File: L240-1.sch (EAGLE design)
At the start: 13 parts, among them IC1 TINY13-20SSU, IC2 LM1117IMPX-3.3, X2 22-23-2021, X3 MKDSN1,5/6-5,08

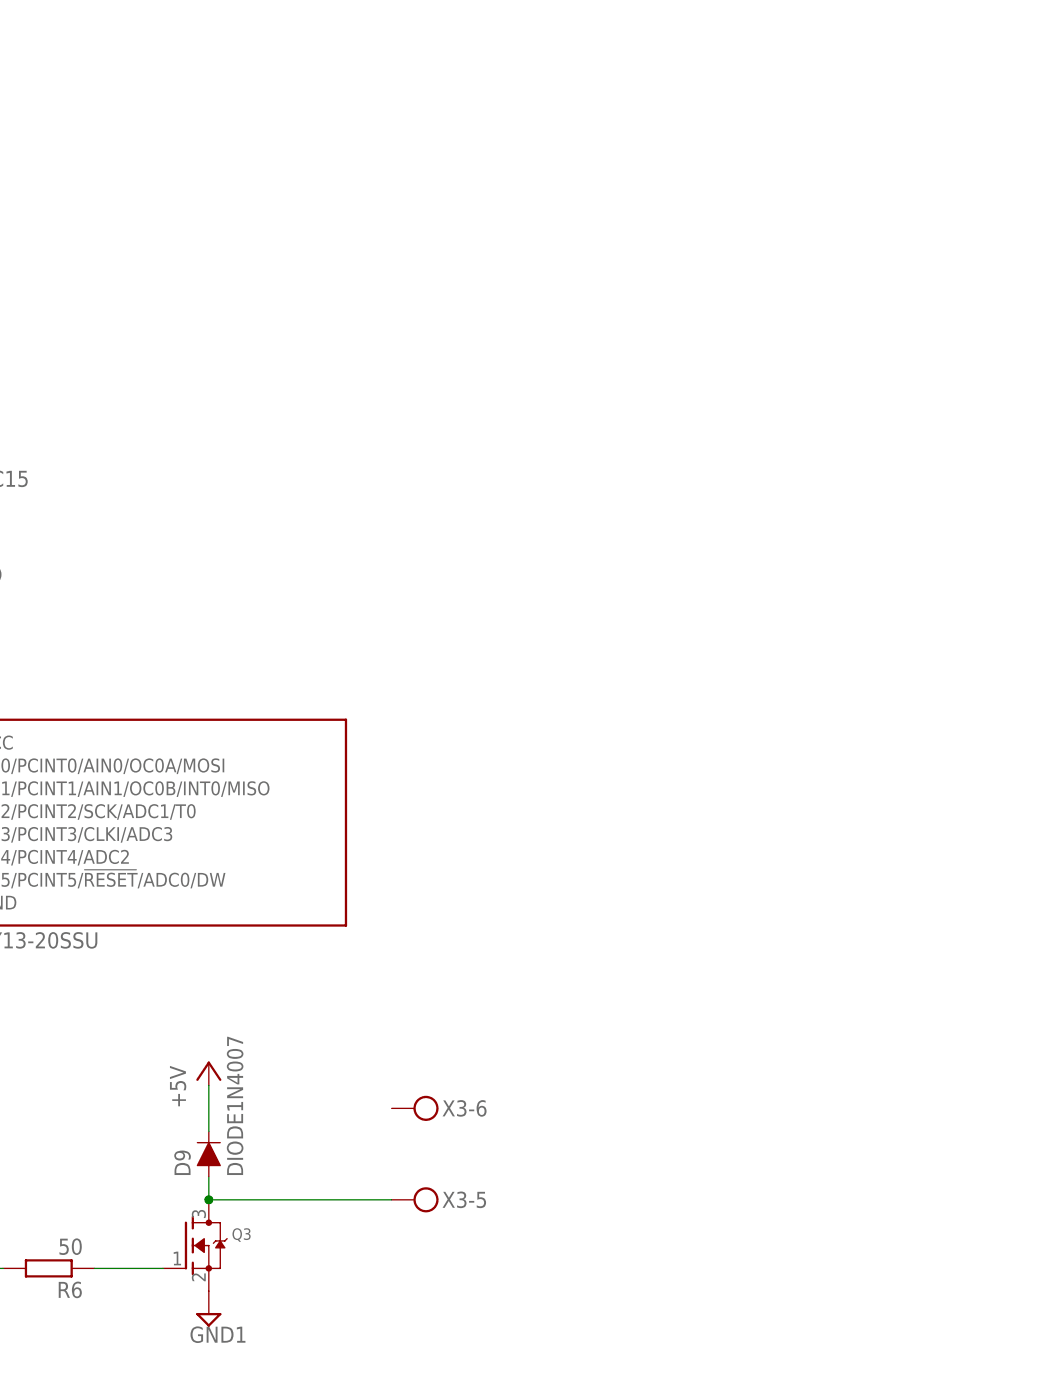
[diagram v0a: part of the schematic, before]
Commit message: relay
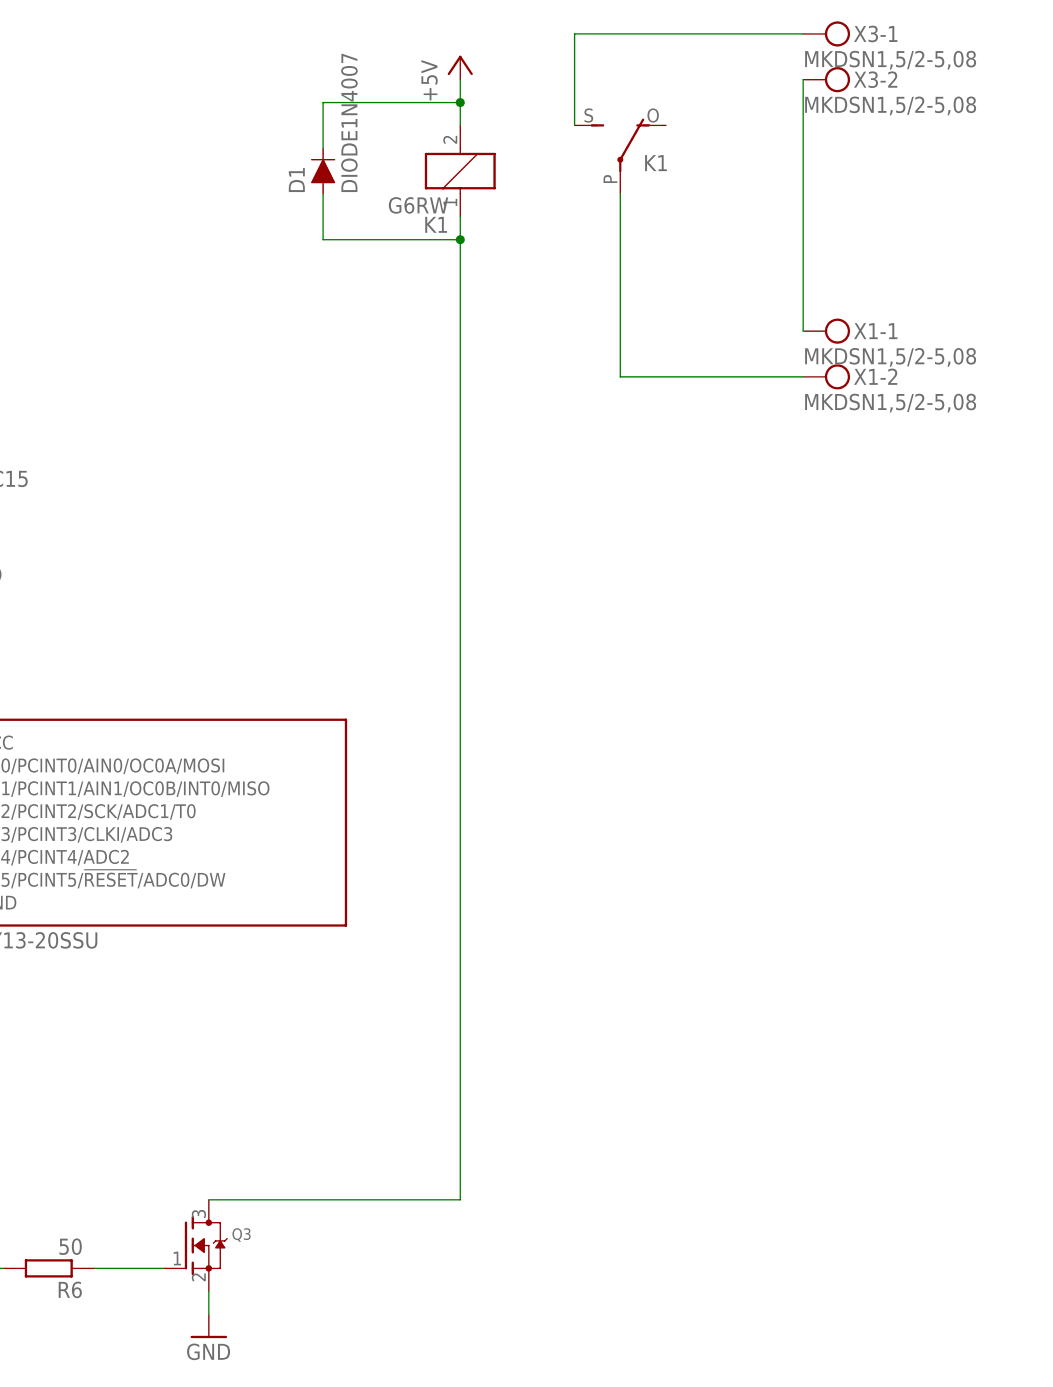
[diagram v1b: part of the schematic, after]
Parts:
- removed D9: DIODE1N4007, MyLib:DIODE1N4007
- added D1: DIODE1N4007, MyLib:DIODE1N4007
- added K1: G6RW, relay:G6RW
- added X1: MKDSN1,5/2-5,08, con-phoenix-508:MKDSN1,5/2-5,08
- X3: value MKDSN1,5/6-5,08 -> MKDSN1,5/2-5,08; device con-phoenix-508:MKDSN1,5/6-5,08 -> con-phoenix-508:MKDSN1,5/2-5,08
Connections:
- removed net GND1: Q3.S
- new net N$1: X1-1.KL, X3-2.KL
- new net N$2: K12.S, X3-1.KL
- new net N$3: K12.P, X1-2.KL
- net +5V: now also D1.C, K11.2; no longer D9.C
- net GND: now also Q3.S
- net N$13: now also D1.A, K11.1; no longer D9.A, X3-5.KL
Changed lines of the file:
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@@
 <part name="IC1" library="atmel" library_urn="urn:adsk.eagle:library:105" deviceset="TINY13" device="SSU" package3d_urn="urn:adsk.eagle:package:4358/1" technology="-20"/>
 <part name="R6" library="rcl" deviceset="R-EU_" device="R0805" value="50"/>
-<part name="X3" library="con-phoenix-508" library_urn="urn:adsk.eagle:library:176" deviceset="MKDSN1,5/6-5,08" device="" package3d_urn="urn:adsk.eagle:package:9634/1"/>
-<part name="D9" library="MyLib" deviceset="DIODE" device="1N4007"/>
 <part name="Q3" library="MyLib" deviceset="MOSFET-N" device="WIDE"/>
-<part name="SUPPLY1" library="supply2" library_urn="urn:adsk.eagle:library:372" deviceset="GND1" device=""/>
 <part name="GND12" library="supply1" deviceset="GND" device=""/>
 <part name="C13" library="rcl" deviceset="C-EU" device="C0805" value="0.1"/>
@@
 <part name="+3V2" library="supply1" deviceset="+3V3" device=""/>
 <part name="GND3" library="supply1" deviceset="GND" device=""/>
-<part name="P+3" library="supply1" deviceset="+5V" device=""/>
 <part name="+3V3" library="supply1" deviceset="+3V3" device=""/>
+<part name="X1" library="con-phoenix-508" library_urn="urn:adsk.eagle:library:176" deviceset="MKDSN1,5/2-5,08" device="" package3d_urn="urn:adsk.eagle:package:9630/1"/>
+<part name="K1" library="relay" library_urn="urn:adsk.eagle:library:339" deviceset="G6RW" device="" package3d_urn="urn:adsk.eagle:package:24332/1"/>
+<part name="X3" library="con-phoenix-508" library_urn="urn:adsk.eagle:library:176" deviceset="MKDSN1,5/2-5,08" device="" package3d_urn="urn:adsk.eagle:package:9630/1"/>
+<part name="P+1" library="supply1" deviceset="+5V" device=""/>
+<part name="D1" library="MyLib" deviceset="DIODE" device="1N4007"/>
+<part name="GND4" library="supply1" deviceset="GND" device=""/>
 </parts>
 <sheets>
@@
 <attribute name="VALUE" x="54.61" y="23.622" size="1.778" layer="96" rot="R180"/>
 </instance>
-<instance part="X3" gate="-5" x="91.44" y="27.94" smashed="yes">
-<attribute name="NAME" x="94.488" y="27.051" size="1.778" layer="95"/>
-</instance>
-<instance part="X3" gate="-6" x="91.44" y="38.1" smashed="yes">
-<attribute name="NAME" x="94.488" y="37.211" size="1.778" layer="95"/>
-</instance>
-<instance part="D9" gate="G$1" x="68.58" y="33.02" smashed="yes" rot="R90">
-<attribute name="NAME" x="66.548" y="30.48" size="1.778" layer="95" font="vector" rot="R90"/>
-<attribute name="VALUE" x="70.612" y="30.48" size="1.778" layer="96" font="vector" rot="R90" align="top-left"/>
-</instance>
 <instance part="Q3" gate="G$1" x="66.04" y="22.86" smashed="yes">
 <attribute name="NAME" x="71.12" y="23.495" size="1.27" layer="95"/>
 <attribute name="VALUE" x="71.12" y="21.59" size="1.27" layer="96"/>
 </instance>
-<instance part="SUPPLY1" gate="G$1" x="68.58" y="15.24" smashed="yes">
-<attribute name="VALUE" x="66.421" y="12.065" size="1.778" layer="96"/>
-</instance>
 <instance part="GND12" gate="1" x="43.18" y="99.06" smashed="yes">
 <attribute name="VALUE" x="40.64" y="96.52" size="1.778" layer="96"/>
@@
 <attribute name="VALUE" x="33.02" y="48.26" size="1.778" layer="96"/>
 </instance>
-<instance part="P+3" gate="1" x="68.58" y="43.18" smashed="yes">
-<attribute name="VALUE" x="66.04" y="38.1" size="1.778" layer="96" rot="R90"/>
-</instance>
 <instance part="+3V3" gate="G$1" x="20.32" y="119.38" smashed="yes">
 <attribute name="VALUE" x="17.78" y="114.3" size="1.778" layer="96" rot="R90"/>
+</instance>
+<instance part="X1" gate="-1" x="137.16" y="124.46" smashed="yes">
+<attribute name="NAME" x="140.208" y="123.571" size="1.778" layer="95"/>
+<attribute name="VALUE" x="134.62" y="120.777" size="1.778" layer="96"/>
+</instance>
+<instance part="X1" gate="-2" x="137.16" y="119.38" smashed="yes">
+<attribute name="NAME" x="140.208" y="118.491" size="1.778" layer="95"/>
+<attribute name="VALUE" x="134.62" y="115.697" size="1.778" layer="96"/>
+</instance>
+<instance part="K1" gate="1" x="96.52" y="142.24" smashed="yes" rot="R180">
+<attribute name="VALUE" x="95.25" y="139.319" size="1.778" layer="96" rot="R180"/>
+<attribute name="PART" x="95.25" y="137.16" size="1.778" layer="95" rot="R180"/>
+</instance>
+<instance part="K1" gate="2" x="114.3" y="142.24" smashed="yes">
+<attribute name="PART" x="116.84" y="142.24" size="1.778" layer="95"/>
+</instance>
+<instance part="X3" gate="-1" x="137.16" y="157.48" smashed="yes">
+<attribute name="NAME" x="140.208" y="156.591" size="1.778" layer="95"/>
+<attribute name="VALUE" x="134.62" y="153.797" size="1.778" layer="96"/>
+</instance>
+<instance part="X3" gate="-2" x="137.16" y="152.4" smashed="yes">
+<attribute name="NAME" x="140.208" y="151.511" size="1.778" layer="95"/>
+<attribute name="VALUE" x="134.62" y="148.717" size="1.778" layer="96"/>
+</instance>
+<instance part="P+1" gate="1" x="96.52" y="154.94" smashed="yes">
+<attribute name="VALUE" x="93.98" y="149.86" size="1.778" layer="96" rot="R90"/>
+</instance>
+<instance part="D1" gate="G$1" x="81.28" y="142.24" smashed="yes" rot="R90">
+<attribute name="NAME" x="79.248" y="139.7" size="1.778" layer="95" font="vector" rot="R90"/>
+<attribute name="VALUE" x="83.312" y="139.7" size="1.778" layer="96" font="vector" rot="R90" align="top-left"/>
+</instance>
+<instance part="GND4" gate="1" x="68.58" y="12.7" smashed="yes">
+<attribute name="VALUE" x="66.04" y="10.16" size="1.778" layer="96"/>
 </instance>
 </instances>
@@
 <net name="N$13" class="0">
 <segment>
-<pinref part="D9" gate="G$1" pin="A"/>
 <pinref part="Q3" gate="G$1" pin="D"/>
-<wire x1="68.58" y1="30.48" x2="68.58" y2="27.94" width="0.1524" layer="91"/>
-<wire x1="68.58" y1="27.94" x2="88.9" y2="27.94" width="0.1524" layer="91"/>
-<junction x="68.58" y="27.94"/>
-<pinref part="X3" gate="-5" pin="KL"/>
-</segment>
-</net>
-<net name="GND1" class="0">
-<segment>
-<pinref part="Q3" gate="G$1" pin="S"/>
-<pinref part="SUPPLY1" gate="G$1" pin="GND1"/>
+<wire x1="68.58" y1="27.94" x2="96.52" y2="27.94" width="0.1524" layer="91"/>
+<pinref part="D1" gate="G$1" pin="A"/>
+<wire x1="96.52" y1="134.62" x2="96.52" y2="27.94" width="0.1524" layer="91"/>
+<wire x1="81.28" y1="139.7" x2="81.28" y2="134.62" width="0.1524" layer="91"/>
+<wire x1="81.28" y1="134.62" x2="96.52" y2="134.62" width="0.1524" layer="91"/>
+<pinref part="K1" gate="1" pin="1"/>
+<wire x1="96.52" y1="134.62" x2="96.52" y2="137.16" width="0.1524" layer="91"/>
+<junction x="96.52" y="134.62"/>
 </segment>
 </net>
@@
 <wire x1="35.56" y1="60.96" x2="35.56" y2="53.34" width="0.1524" layer="91"/>
 </segment>
+<segment>
+<pinref part="GND4" gate="1" pin="GND"/>
+<pinref part="Q3" gate="G$1" pin="S"/>
+<wire x1="68.58" y1="15.24" x2="68.58" y2="17.78" width="0.1524" layer="91"/>
+</segment>
 </net>
 <net name="+5V" class="0">
@@
 </segment>
 <segment>
-<pinref part="D9" gate="G$1" pin="C"/>
-<pinref part="P+3" gate="1" pin="+5V"/>
-<wire x1="68.58" y1="35.56" x2="68.58" y2="40.64" width="0.1524" layer="91"/>
+<pinref part="K1" gate="1" pin="2"/>
+<pinref part="P+1" gate="1" pin="+5V"/>
+<wire x1="96.52" y1="147.32" x2="96.52" y2="149.86" width="0.1524" layer="91"/>
+<pinref part="D1" gate="G$1" pin="C"/>
+<wire x1="96.52" y1="149.86" x2="96.52" y2="152.4" width="0.1524" layer="91"/>
+<wire x1="96.52" y1="149.86" x2="81.28" y2="149.86" width="0.1524" layer="91"/>
+<wire x1="81.28" y1="149.86" x2="81.28" y2="144.78" width="0.1524" layer="91"/>
+<junction x="96.52" y="149.86"/>
 </segment>
 </net>
@@
 </segment>
 </net>
+<net name="N$1" class="0">
+<segment>
+<pinref part="X1" gate="-1" pin="KL"/>
+<pinref part="X3" gate="-2" pin="KL"/>
+<wire x1="134.62" y1="124.46" x2="134.62" y2="152.4" width="0.1524" layer="91"/>
+</segment>
+</net>
+<net name="N$2" class="0">
+<segment>
+<pinref part="X3" gate="-1" pin="KL"/>
+<pinref part="K1" gate="2" pin="S"/>
+<wire x1="134.62" y1="157.48" x2="109.22" y2="157.48" width="0.1524" layer="91"/>
+<wire x1="109.22" y1="157.48" x2="109.22" y2="147.32" width="0.1524" layer="91"/>
+</segment>
+</net>
+<net name="N$3" class="0">
+<segment>
+<pinref part="K1" gate="2" pin="P"/>
+<pinref part="X1" gate="-2" pin="KL"/>
+<wire x1="114.3" y1="139.7" x2="114.3" y2="119.38" width="0.1524" layer="91"/>
+<wire x1="114.3" y1="119.38" x2="134.62" y2="119.38" width="0.1524" layer="91"/>
+</segment>
+</net>
